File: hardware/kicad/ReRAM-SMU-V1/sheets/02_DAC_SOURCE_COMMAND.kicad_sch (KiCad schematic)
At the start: 38 parts, among them U1 AD5764CSUZ PRIMARY 5V ref 20V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, U2 ADA4522-1 VCSRC conditioning 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, U3 ADA4522-1 VCSNK conditioning 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

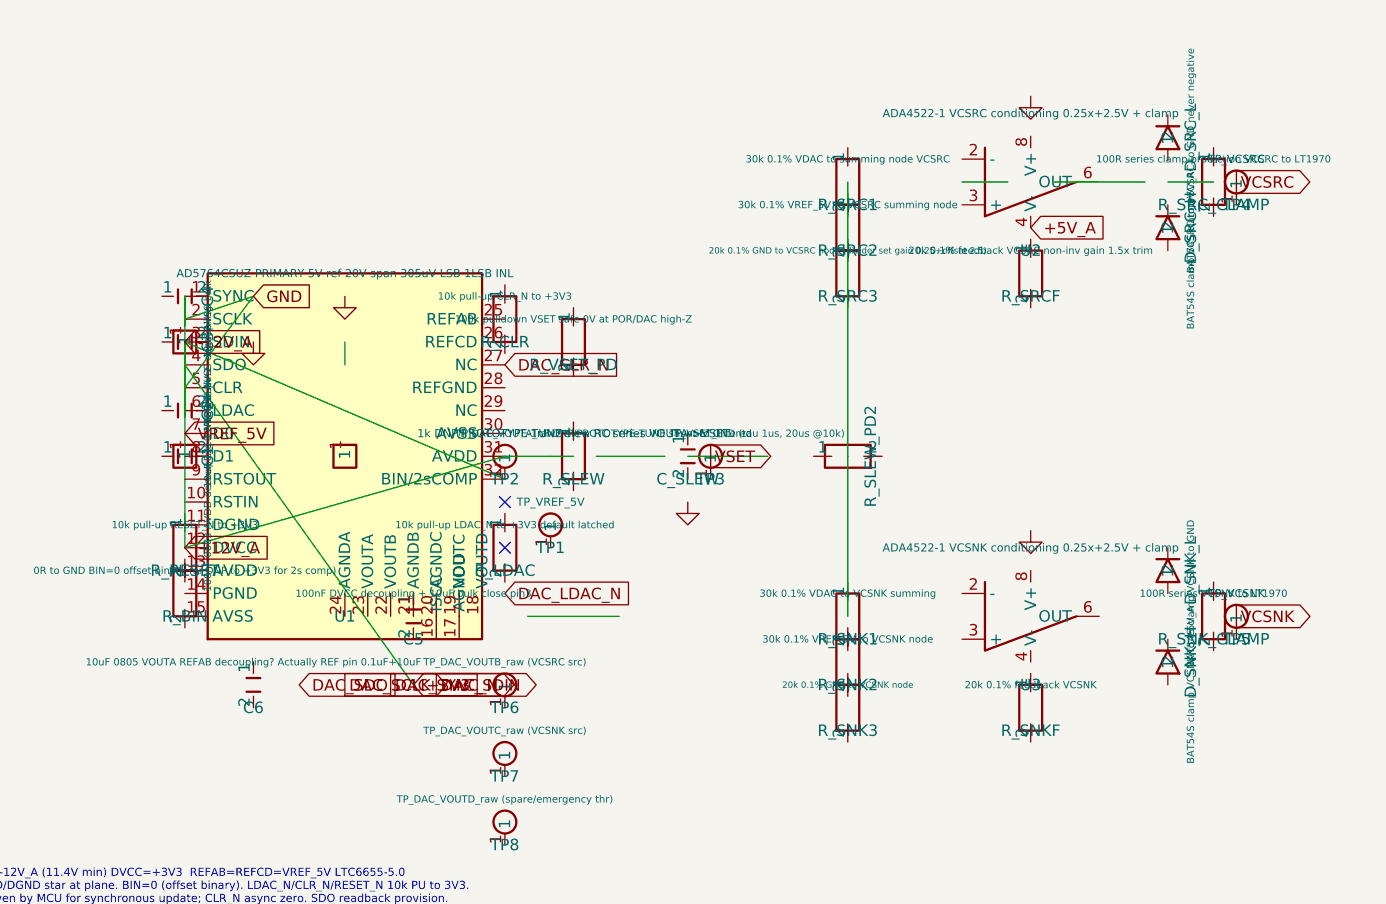
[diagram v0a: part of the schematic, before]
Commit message: Beta
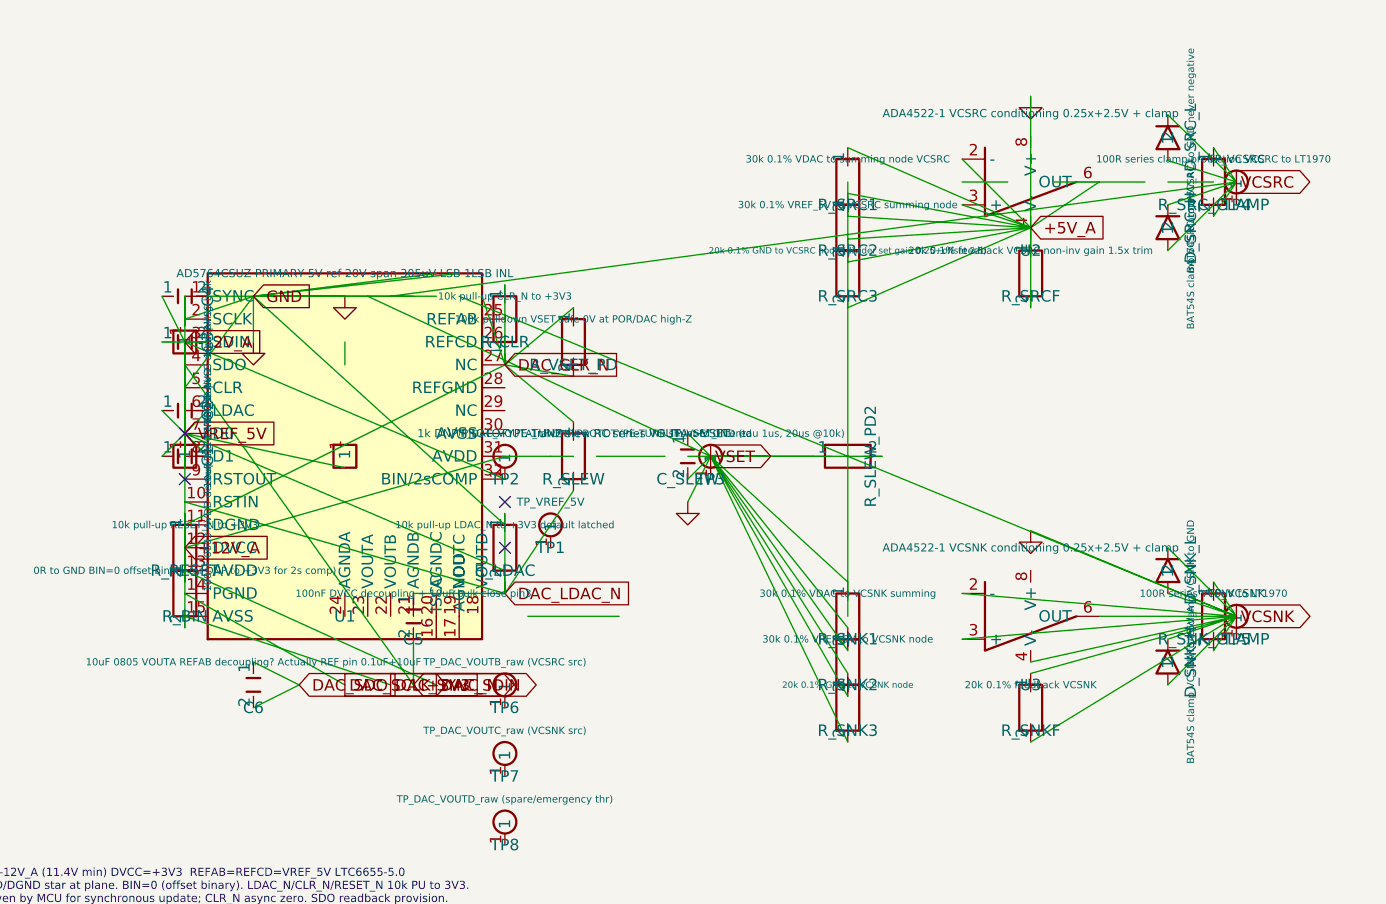
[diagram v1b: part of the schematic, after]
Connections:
- net +12V_A: now also C1.1, C1.2, C2.1, C2.2, C3.1, C3.2, C4.1, C4.2, C5.2, D_SRC_H.1, D_SRC_H.2, R_BIN.1, R_BIN.2, U1.6 (LDAC)
- net +5V_A: now also R_SRC1.1, R_SRC1.2, R_SRC2.1, R_SRC2.2, R_SRC3.1, R_SRC3.2, R_SRCF.1, R_SRCF.2, U2.2 (-), U2.3 (+), U2.6 (OUT)
- net DAC_CLR_N: now also R_CLR.1, R_CLR.2, R_SLEW.1, R_VSET_PD.1, R_VSET_PD.2, U1.11 (DGND)
- net DAC_LDAC_N: now also C5.1, R_LDAC.1, R_LDAC.2, R_SLEW.2, U1.10 (RSTIN)
- net DAC_SCLK: now also U1.14 (PGND)
- net DAC_SDIN: now also U1.13 (AVDD)
- net DAC_SDO: now also C6.1, C6.2
- net DAC_SYNC_N: now also U1.15 (AVSS)
- net VCSNK: now also D_SNK_H.1, D_SNK_H.2, D_SNK_L.1, D_SNK_L.2, R_SNKF.1, R_SNKF.2, R_SNK_CLAMP.1, R_SNK_CLAMP.2, U3.2 (-), U3.3 (+), U3.4 (V-), U3.6 (OUT)
- net VCSRC: now also D_SRC_H.1, D_SRC_H.2, D_SRC_L.1, D_SRC_L.2, R_SRC_CLAMP.1, R_SRC_CLAMP.2
- net VSET: now also C_SLEW.1, C_SLEW.2, R_SLEW_PD2.1, R_SLEW_PD2.2, R_SNK1.1, R_SNK1.2, R_SNK2.1, R_SNK2.2, R_SNK3.1, R_SNK3.2
- no-connect marks 2 -> 4
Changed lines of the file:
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@@
 	(wire (pts (xy 33.019999999999996 55.88) (xy 40.64 45.72)) (stroke (width 0) (type default)) (uuid "wire-pwr-11-50.8"))
 	(wire (pts (xy 33.019999999999996 48.26) (xy 40.64 45.72)) (stroke (width 0) (type default)) (uuid "wire-pwr-14-50.8"))
+	(wire (pts (xy 33.020 81.280) (xy 55.880 88.900)) (stroke (width 0) (type default)))
+	(wire (pts (xy 33.020 78.740) (xy 50.800 88.900)) (stroke (width 0) (type default)))
+	(wire (pts (xy 33.020 76.200) (xy 60.960 88.900)) (stroke (width 0) (type default)))
+	(wire (pts (xy 33.020 71.120) (xy 68.580 53.340)) (stroke (width 0) (type default)))
+	(wire (pts (xy 33.020 68.580) (xy 68.580 78.740)) (stroke (width 0) (type default)))
+	(wire (pts (xy 33.020 58.420) (xy 33.020 60.960)) (stroke (width 0) (type default)))
+	(wire (pts (xy 60.960 43.180) (xy 40.640 45.720)) (stroke (width 0) (type default)))
+	(wire (pts (xy 63.500 43.180) (xy 40.640 45.720)) (stroke (width 0) (type default)))
+	(wire (pts (xy 66.040 45.720) (xy 68.580 53.340)) (stroke (width 0) (type default)))
+	(wire (pts (xy 63.500 45.720) (xy 149.860 81.280)) (stroke (width 0) (type default)))
+	(wire (pts (xy 60.960 45.720) (xy 40.640 45.720)) (stroke (width 0) (type default)))
+	(wire (pts (xy 58.420 45.720) (xy 40.640 45.720)) (stroke (width 0) (type default)))
+	(wire (pts (xy 55.880 45.720) (xy 149.860 33.020)) (stroke (width 0) (type default)))
+	(wire (pts (xy 53.340 45.720) (xy 91.440 63.500)) (stroke (width 0) (type default)))
+	(wire (pts (xy 50.800 45.720) (xy 40.640 45.720)) (stroke (width 0) (type default)))
+	(wire (pts (xy 68.580 76.200) (xy 33.020 60.960)) (stroke (width 0) (type default)))
+	(wire (pts (xy 68.580 71.120) (xy 40.640 45.720)) (stroke (width 0) (type default)))
+	(wire (pts (xy 30.480 63.500) (xy 33.020 60.960)) (stroke (width 0) (type default)))
+	(wire (pts (xy 35.560 63.500) (xy 33.020 60.960)) (stroke (width 0) (type default)))
+	(wire (pts (xy 30.480 58.420) (xy 33.020 60.960)) (stroke (width 0) (type default)))
+	(wire (pts (xy 35.560 58.420) (xy 33.020 60.960)) (stroke (width 0) (type default)))
+	(wire (pts (xy 30.480 50.800) (xy 33.020 50.800)) (stroke (width 0) (type default)))
+	(wire (pts (xy 35.560 50.800) (xy 33.020 50.800)) (stroke (width 0) (type default)))
+	(wire (pts (xy 30.480 45.720) (xy 33.020 50.800)) (stroke (width 0) (type default)))
+	(wire (pts (xy 35.560 45.720) (xy 40.640 45.720)) (stroke (width 0) (type default)))
+	(wire (pts (xy 58.420 83.820) (xy 58.420 88.900)) (stroke (width 0) (type default)))
+	(wire (pts (xy 58.420 78.740) (xy 68.580 78.740)) (stroke (width 0) (type default)))
+	(wire (pts (xy 40.640 91.440) (xy 45.720 88.900)) (stroke (width 0) (type default)))
+	(wire (pts (xy 40.640 86.360) (xy 45.720 88.900)) (stroke (width 0) (type default)))
+	(wire (pts (xy 68.580 77.470) (xy 68.580 78.740)) (stroke (width 0) (type default)))
+	(wire (pts (xy 68.580 69.850) (xy 68.580 78.740)) (stroke (width 0) (type default)))
+	(wire (pts (xy 68.580 52.070) (xy 68.580 53.340)) (stroke (width 0) (type default)))
+	(wire (pts (xy 68.580 44.450) (xy 68.580 53.340)) (stroke (width 0) (type default)))
+	(wire (pts (xy 33.020 77.470) (xy 33.020 73.660)) (stroke (width 0) (type default)))
+	(wire (pts (xy 33.020 69.850) (xy 33.020 73.660)) (stroke (width 0) (type default)))
+	(wire (pts (xy 33.020 82.550) (xy 33.020 73.660)) (stroke (width 0) (type default)))
+	(wire (pts (xy 33.020 74.930) (xy 33.020 73.660)) (stroke (width 0) (type default)))
+	(wire (pts (xy 76.200 67.310) (xy 68.580 78.740)) (stroke (width 0) (type default)))
+	(wire (pts (xy 76.200 59.690) (xy 68.580 53.340)) (stroke (width 0) (type default)))
+	(wire (pts (xy 88.900 66.040) (xy 91.440 63.500)) (stroke (width 0) (type default)))
+	(wire (pts (xy 88.900 60.960) (xy 91.440 63.500)) (stroke (width 0) (type default)))
+	(wire (pts (xy 76.200 54.610) (xy 68.580 53.340)) (stroke (width 0) (type default)))
+	(wire (pts (xy 76.200 46.990) (xy 68.580 53.340)) (stroke (width 0) (type default)))
+	(wire (pts (xy 119.380 35.560) (xy 127.000 38.100)) (stroke (width 0) (type default)))
+	(wire (pts (xy 119.380 30.480) (xy 127.000 38.100)) (stroke (width 0) (type default)))
+	(wire (pts (xy 134.620 33.020) (xy 127.000 38.100)) (stroke (width 0) (type default)))
+	(wire (pts (xy 127.000 38.100) (xy 127.000 38.100)) (stroke (width 0) (type default)))
+	(wire (pts (xy 119.380 83.820) (xy 149.860 81.280)) (stroke (width 0) (type default)))
+	(wire (pts (xy 119.380 78.740) (xy 149.860 81.280)) (stroke (width 0) (type default)))
+	(wire (pts (xy 134.620 81.280) (xy 149.860 81.280)) (stroke (width 0) (type default)))
+	(wire (pts (xy 127.000 86.360) (xy 149.860 81.280)) (stroke (width 0) (type default)))
+	(wire (pts (xy 106.680 36.830) (xy 127.000 38.100)) (stroke (width 0) (type default)))
+	(wire (pts (xy 106.680 29.210) (xy 127.000 38.100)) (stroke (width 0) (type default)))
+	(wire (pts (xy 106.680 41.910) (xy 127.000 38.100)) (stroke (width 0) (type default)))
+	(wire (pts (xy 106.680 34.290) (xy 127.000 38.100)) (stroke (width 0) (type default)))
+	(wire (pts (xy 106.680 46.990) (xy 127.000 38.100)) (stroke (width 0) (type default)))
+	(wire (pts (xy 106.680 39.370) (xy 127.000 38.100)) (stroke (width 0) (type default)))
+	(wire (pts (xy 127.000 46.990) (xy 127.000 38.100)) (stroke (width 0) (type default)))
+	(wire (pts (xy 127.000 39.370) (xy 127.000 38.100)) (stroke (width 0) (type default)))
+	(wire (pts (xy 147.320 36.830) (xy 149.860 33.020)) (stroke (width 0) (type default)))
+	(wire (pts (xy 147.320 29.210) (xy 149.860 33.020)) (stroke (width 0) (type default)))
+	(wire (pts (xy 142.240 35.560) (xy 149.860 33.020)) (stroke (width 0) (type default)))
+	(wire (pts (xy 142.240 40.640) (xy 149.860 33.020)) (stroke (width 0) (type default)))
+	(wire (pts (xy 142.240 25.560) (xy 149.860 33.020)) (stroke (width 0) (type default)))
+	(wire (pts (xy 142.240 30.640) (xy 149.860 33.020)) (stroke (width 0) (type default)))
+	(wire (pts (xy 106.680 85.090) (xy 91.440 63.500)) (stroke (width 0) (type default)))
+	(wire (pts (xy 106.680 77.470) (xy 91.440 63.500)) (stroke (width 0) (type default)))
+	(wire (pts (xy 106.680 90.170) (xy 91.440 63.500)) (stroke (width 0) (type default)))
+	(wire (pts (xy 106.680 82.550) (xy 91.440 63.500)) (stroke (width 0) (type default)))
+	(wire (pts (xy 106.680 95.250) (xy 91.440 63.500)) (stroke (width 0) (type default)))
+	(wire (pts (xy 106.680 87.630) (xy 91.440 63.500)) (stroke (width 0) (type default)))
+	(wire (pts (xy 127.000 95.250) (xy 149.860 81.280)) (stroke (width 0) (type default)))
+	(wire (pts (xy 127.000 87.630) (xy 149.860 81.280)) (stroke (width 0) (type default)))
+	(wire (pts (xy 147.320 85.090) (xy 149.860 81.280)) (stroke (width 0) (type default)))
+	(wire (pts (xy 147.320 77.470) (xy 149.860 81.280)) (stroke (width 0) (type default)))
+	(wire (pts (xy 142.240 83.820) (xy 149.860 81.280)) (stroke (width 0) (type default)))
+	(wire (pts (xy 142.240 88.900) (xy 149.860 81.280)) (stroke (width 0) (type default)))
+	(wire (pts (xy 142.240 73.660) (xy 149.860 81.280)) (stroke (width 0) (type default)))
+	(wire (pts (xy 142.240 78.740) (xy 149.860 81.280)) (stroke (width 0) (type default)))
+	(wire (pts (xy 102.870 63.500) (xy 91.440 63.500)) (stroke (width 0) (type default)))
+	(wire (pts (xy 110.490 63.500) (xy 91.440 63.500)) (stroke (width 0) (type default)))
+	(wire (pts (xy 40.640 50.800) (xy 40.640 45.720)) (stroke (width 0) (type default)))
+	(wire (pts (xy 88.900 68.580) (xy 91.440 63.500)) (stroke (width 0) (type default)))
+	(wire (pts (xy 127.000 23.500) (xy 127.000 38.100)) (stroke (width 0) (type default)))
+	(wire (pts (xy 127.000 71.760) (xy 149.860 81.280)) (stroke (width 0) (type default)))
+	(wire (pts (xy 33.020 64.770) (xy 33.020 60.960)) (stroke (width 0) (type default)))
+	(wire (pts (xy 33.020 52.070) (xy 33.020 50.800)) (stroke (width 0) (type default)))
+	(wire (pts (xy 50.800 64.770) (xy 33.020 60.960)) (stroke (width 0) (type default)))
+	(no_connect (at 33.020 66.040))
+	(no_connect (at 33.020 60.960))
 )
